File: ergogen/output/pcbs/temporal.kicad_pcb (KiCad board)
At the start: 2 copper layers, 144.2 x 91.9 mm, 55 parts

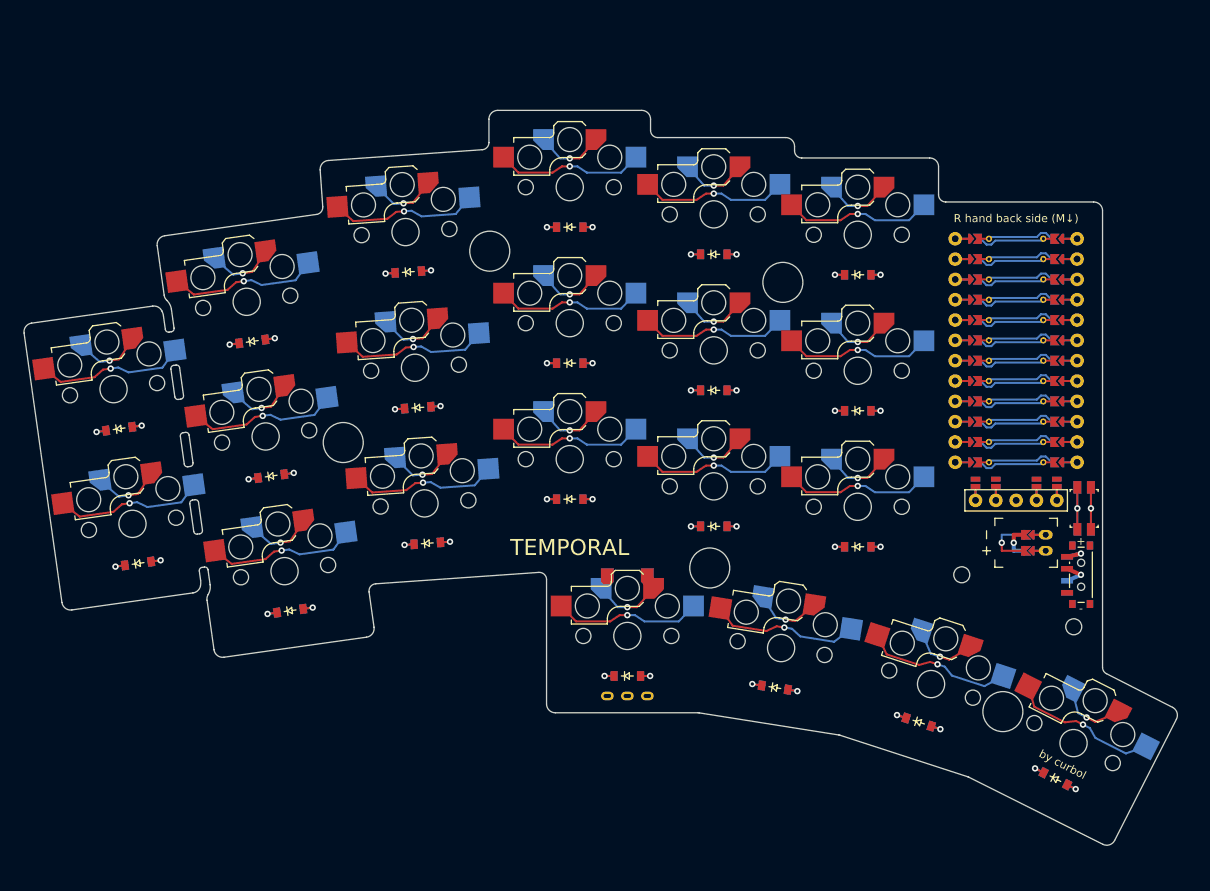
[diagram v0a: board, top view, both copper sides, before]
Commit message: new shape
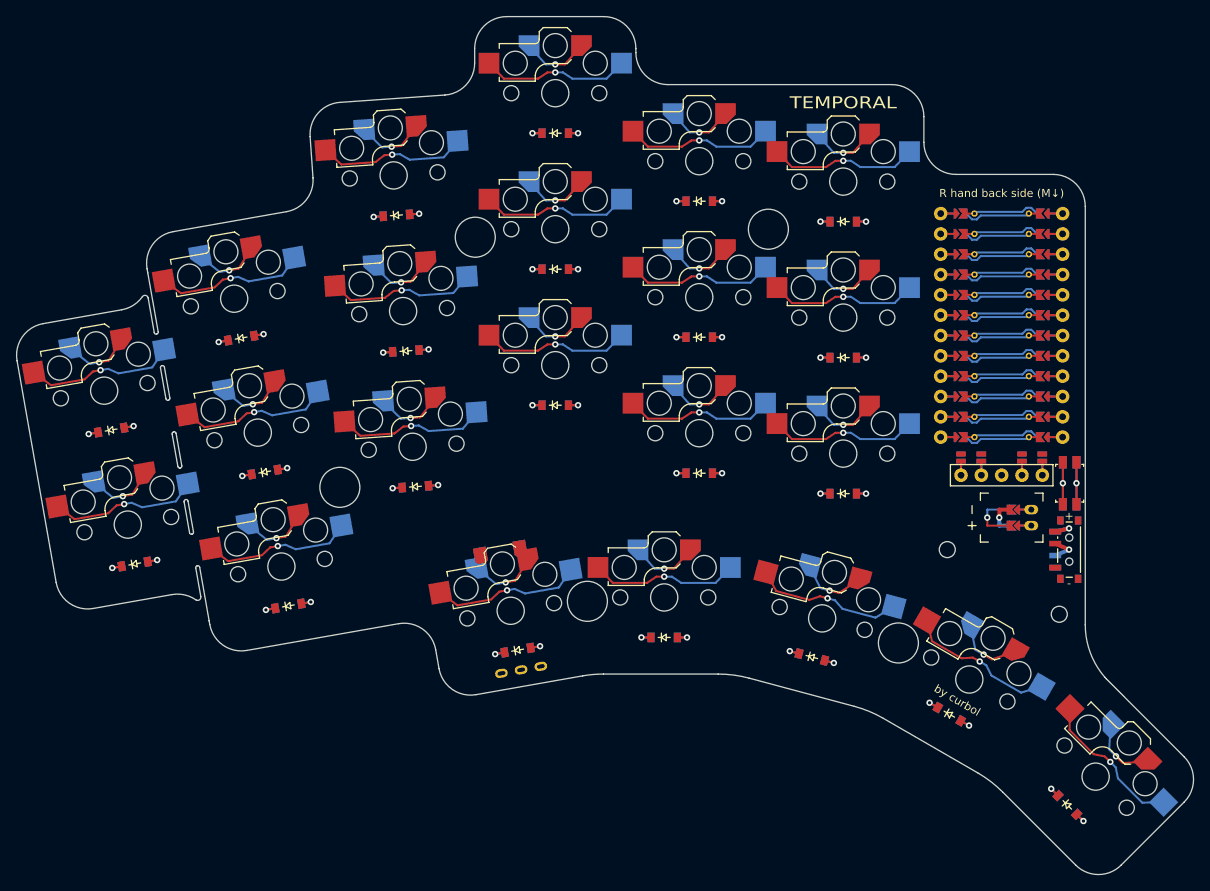
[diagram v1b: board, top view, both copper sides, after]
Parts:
- added D22: , ceoloide:diode_tht_sod123, F.Cu at (164.5, 118.3)
- added S22: , ceoloide:switch_choc_v1_v2, B.Cu at (168.0, 114.8)
- moved S19 15.9 mm to (114.1, 92.4), turned to 0 degrees
- moved S20 15.9 mm to (133.8, 95.0), turned to -15 degrees
- moved MH4 15.9 mm to (104.5, 92.8), turned to 10 degrees
- moved D20 15.6 mm to (132.5, 99.8), turned to -15 degrees
- moved MH3 15.6 mm to (143.4, 98.1), turned to -15 degrees
- moved D21 15.5 mm to (149.7, 107.0), turned to -30 degrees
- moved S21 15.3 mm to (152.2, 102.6), turned to -30 degrees
- moved D19 15.2 mm to (114.1, 97.4), turned to 0 degrees
- moved RE1 14.9 mm to (94.9, 94.0), turned to 10 degrees
- moved S18 14.9 mm to (94.9, 94.0), turned to 10 degrees
- moved D18 14.1 mm to (95.8, 99.0), turned to 10 degrees
- moved D10 11.9 mm to (100.5, 51.3)
- moved D11 11.9 mm to (100.5, 34.3)
- moved D9 11.9 mm to (100.5, 68.3)
- moved S10 11.9 mm to (100.5, 46.3)
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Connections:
- RE1 pad S1: col_ring -> col_pinky
- S18 pad 2: col_ring -> col_pinky
- S19 pad 2: col_middle -> col_ring
- S20 pad 2: col_index -> col_middle
- S21 pad 2: col_inner -> col_index
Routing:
- net col_pinky: track 56.0 -> 74.7 mm, vias 3 -> 4
- net extra_thumb: track 0.00 -> 11.1 mm, vias 0 -> 2
- net row_thumb: track 9.60 -> 12.0 mm, vias 4 -> 5
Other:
- board size 144.2 x 91.9 mm -> 147.1 x 107.2 mm
